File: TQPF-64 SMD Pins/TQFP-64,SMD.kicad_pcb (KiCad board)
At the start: 2 copper layers, 3 parts, among them J1 Conn_02x32_Counter_Clockwise, J2 Conn_01x32, J3 Conn_01x32

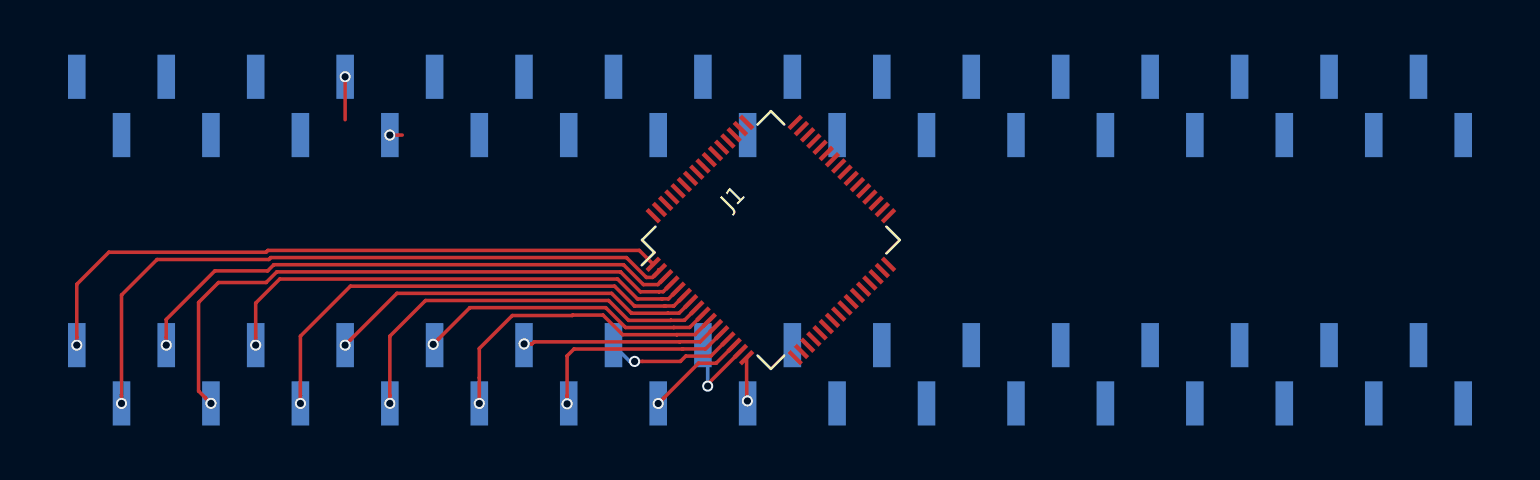
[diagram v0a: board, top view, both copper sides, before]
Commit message: Initial Commit
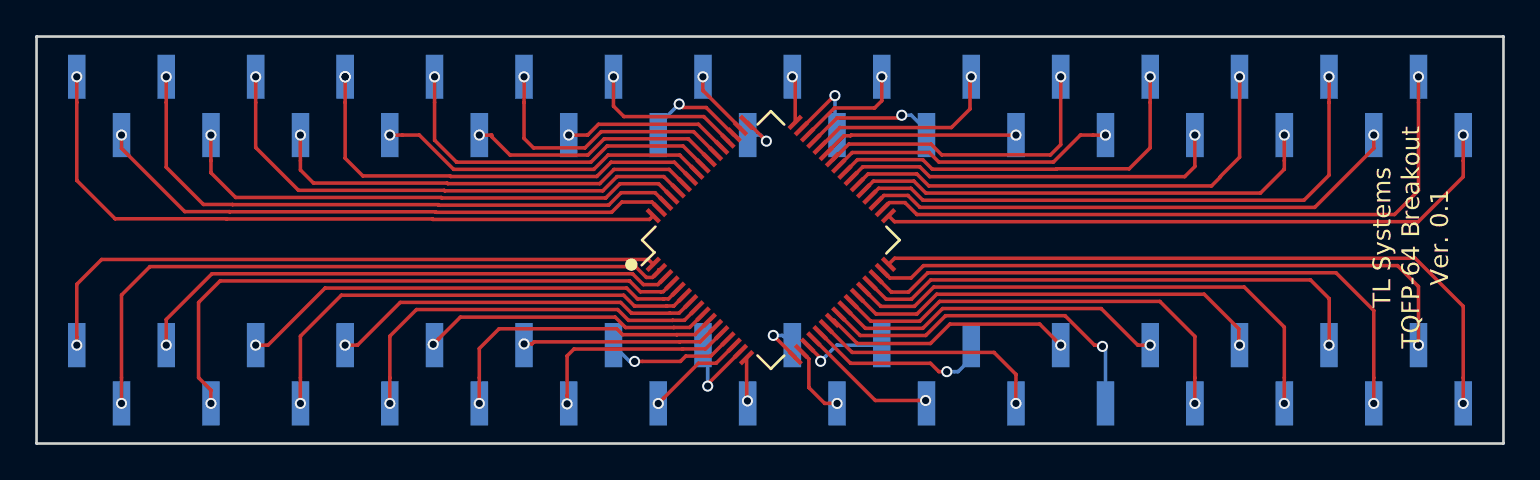
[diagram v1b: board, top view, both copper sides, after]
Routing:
- net Net-(J1-Pad64): track 0.00 -> 39.6 mm, vias 0 -> 1
- net Net-(J1-Pad32): track 0.00 -> 39.4 mm, vias 0 -> 1
- net Net-(J1-Pad34): track 0.00 -> 37.9 mm, vias 0 -> 1
- net Net-(J1-Pad33): track 0.00 -> 36.2 mm, vias 0 -> 1
- net Net-(J1-Pad30): track 0.00 -> 35.2 mm, vias 0 -> 1
- net Net-(J1-Pad62): track 0.00 -> 34.9 mm, vias 0 -> 1
- net Net-(J1-Pad31): track 0.00 -> 34.7 mm, vias 0 -> 1
- net Net-(J1-Pad63): track 0.00 -> 33.2 mm, vias 0 -> 1
- net Net-(J1-Pad36): track 0.00 -> 32.7 mm, vias 0 -> 1
- net Net-(J1-Pad35): track 0.00 -> 30.9 mm, vias 0 -> 1
- net Net-(J1-Pad28): track 0.00 -> 30.0 mm, vias 0 -> 1
- net Net-(J1-Pad29): track 0.00 -> 30.0 mm, vias 0 -> 1
- net Net-(J1-Pad60): track 0.00 -> 29.7 mm, vias 0 -> 1
- net Net-(J1-Pad61): track 0.00 -> 29.6 mm, vias 0 -> 1
- net Net-(J1-Pad38): track 0.00 -> 27.5 mm, vias 0 -> 1
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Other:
- board outline added: 83.3 x 23.1 mm
- board text added: "TL Systems TQFP-64 Breakout Ver. 0.1"
